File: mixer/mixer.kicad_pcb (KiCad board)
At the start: 2 copper layers, 39 parts, among them J1 IN1, J2 IN1, J3 IN1, J4 IN1, J5 IN1, J6 IN1, J7 IN1, J8 Conn_02x05_Odd_Even, Q1 Q_NPN_CBE, U1 TL074

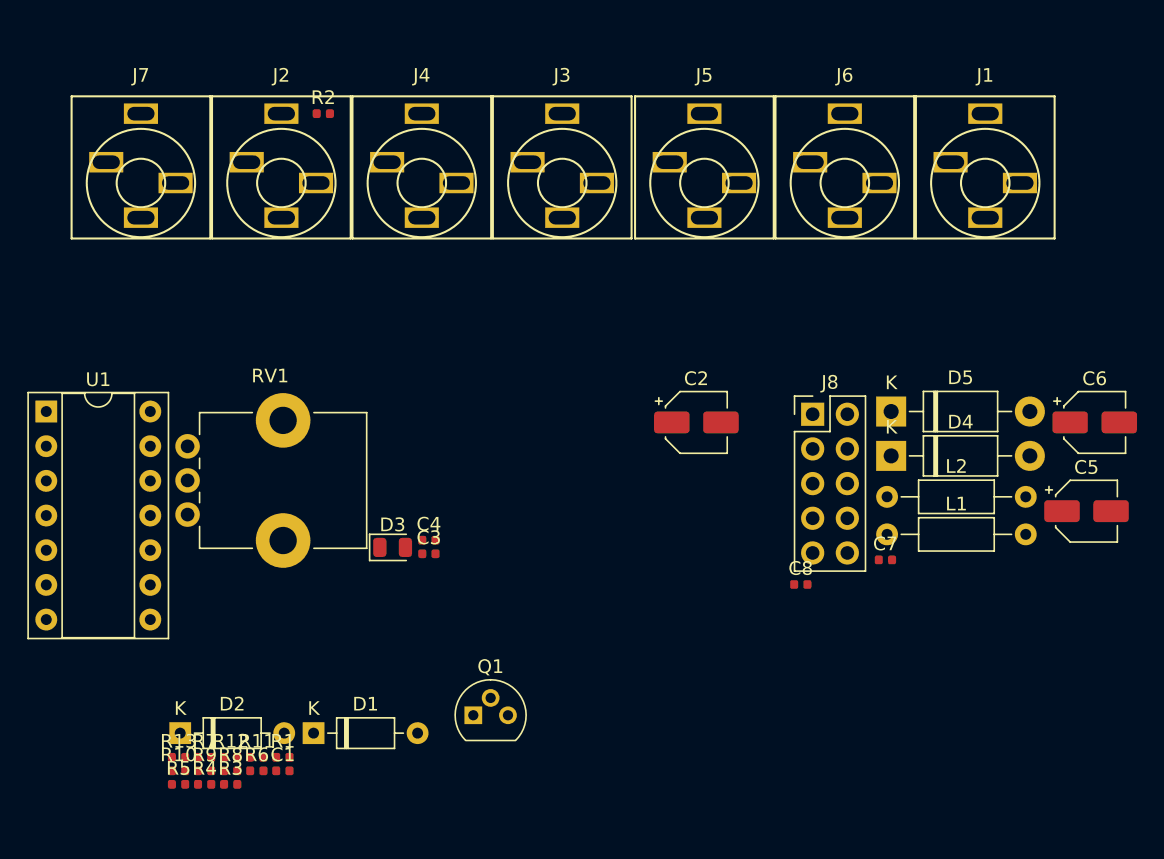
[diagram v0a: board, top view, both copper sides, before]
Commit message: Gerber mixer
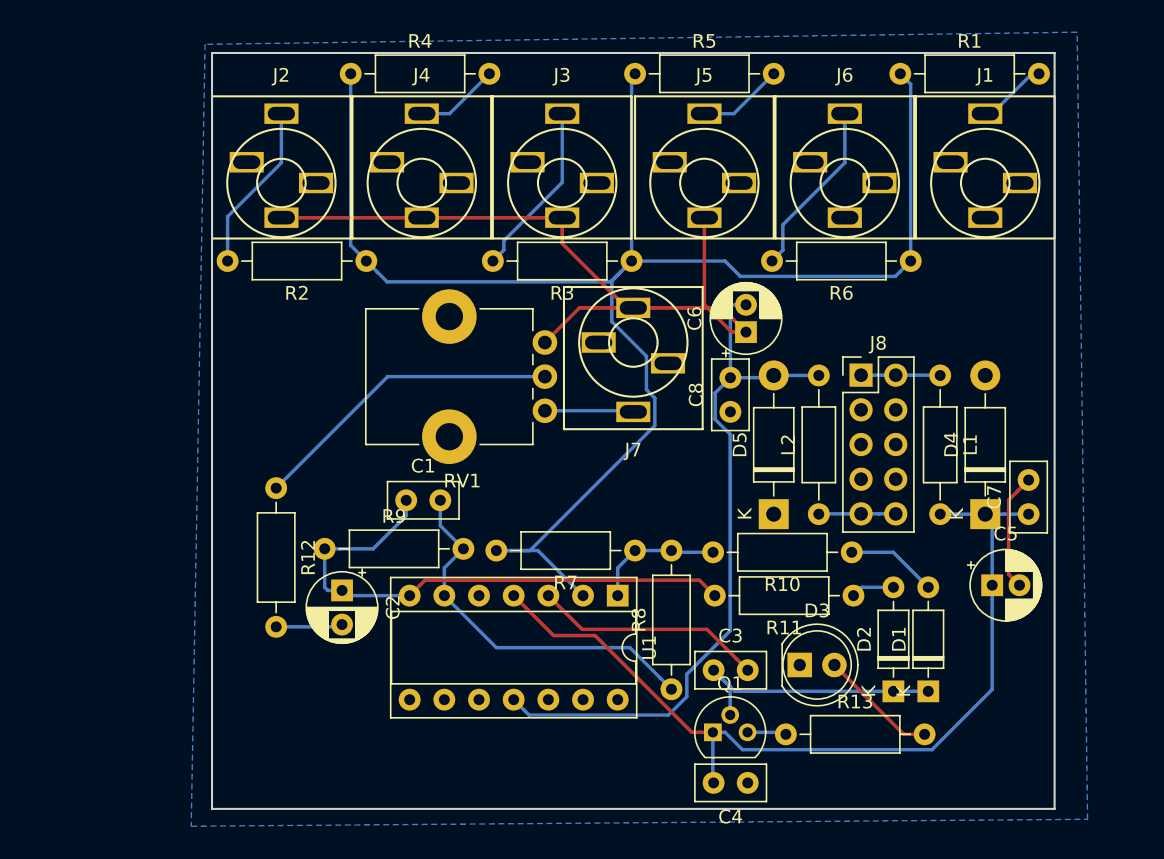
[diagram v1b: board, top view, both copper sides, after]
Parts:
- C1, C3, C4, C7, C8: footprint Capacitor_SMD:C_0402_1005Metric -> Capacitor_THT:C_Disc_D5.0mm_W2.5mm_P2.50mm
- C2: footprint Capacitor_SMD:CP_Elec_4x5.3 -> Capacitor_THT:CP_Radial_D5.0mm_P2.50mm
- C5, C6: footprint Capacitor_SMD:CP_Elec_4x5.3 -> Capacitor_THT:CP_Radial_D5.0mm_P2.00mm
- D3: footprint LED_SMD:LED_0805_2012Metric -> LED_THT:LED_D5.0mm
- J7: value IN1 -> OUT1
- Q1: value Q_NPN_CBE -> BC546a
- R1, R12, R13, R2, R3, R4, R5, R6, R7, R8, R9: footprint Resistor_SMD:R_0402_1005Metric -> Resistor_THT:R_Axial_DIN0207_L6.3mm_D2.5mm_P10.16mm_Horizontal
- R10, R11: value 8k -> 8k2; footprint Resistor_SMD:R_0402_1005Metric -> Resistor_THT:R_Axial_DIN0207_L6.3mm_D2.5mm_P10.16mm_Horizontal
- moved R1 67.5 mm to (110.7, 16.4)
- moved R5 61.9 mm to (91.3, 16.4)
- moved R6 60.7 mm to (111.5, 30.1), turned to 180 degrees
- moved R4 53.1 mm to (70.5, 16.4)
- moved D2 52.3 mm to (110.2, 61.6), turned to 90 degrees
- moved R10 51.8 mm to (107.2, 51.4), turned to 180 degrees
- moved R3 48.3 mm to (91.1, 30.1), turned to 180 degrees
- moved R11 45.3 mm to (107.3, 54.6), turned to 180 degrees
- moved D1 45.1 mm to (112.8, 61.6), turned to 90 degrees
- moved R13 44.5 mm to (102.4, 64.8)
- moved U1 44.0 mm to (90.0, 54.6), turned to 270 degrees
- moved J7 37.9 mm to (91.2, 36.1), turned to 180 degrees
- moved R7 35.0 mm to (91.3, 51.3), turned to 180 degrees
- moved R8 32.8 mm to (94.0, 61.5), turned to 90 degrees
- moved D3 31.0 mm to (103.4, 59.7)
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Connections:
- J8 pad 1: 12V -> 12VC
- J8 pad 10: -12V -> -12VC
- J8 pad 2: 12V -> 12VC
- J8 pad 9: -12V -> -12VC
- L1 pad 1: 12V -> 12VC
- L2 pad 1: -12V -> -12VC
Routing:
- net mixed: track 0.00 -> 121.2 mm
- net GND: track 0.00 -> 81.9 mm
- net 12V: track 0.00 -> 64.8 mm
- net -12V: track 0.00 -> 52.3 mm
- net Net-(C1-Pad1): track 0.00 -> 40.7 mm
- net Net-(C1-Pad2): track 0.00 -> 27.7 mm
- net Net-(R12-Pad1): track 0.00 -> 23.1 mm
- net Net-(C3-Pad1): track 0.00 -> 20.1 mm
- net Net-(J6-PadT): track 0.00 -> 13.0 mm
- net Net-(J3-PadT): track 0.00 -> 12.9 mm
- net Net-(J2-PadT): track 0.00 -> 12.4 mm
- net Net-(R10-Pad2): track 0.00 -> 9.60 mm
- net Net-(D3-Pad2): track 0.00 -> 8.71 mm
- net Net-(D1-Pad2): track 0.00 -> 6.66 mm
- net Net-(J7-PadT): track 0.00 -> 6.51 mm
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- added copper zone on B.Cu, net GND
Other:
- board outline added: 61.7 x 55.4 mm
